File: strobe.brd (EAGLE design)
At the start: 160 x 100 mm, 67 parts, among them IC1 AT90USB162A, Q1 IRF3704S, Q2 IRF3704S, Q4 IRF3704S, Q5 IRF3704S, T1 BC849, T2 BC849, T3 BC849, T4 BC849, T5 BC849, T6 BC849, T7 BC849, T8 BC849, X6 RJ45-6LC21-B

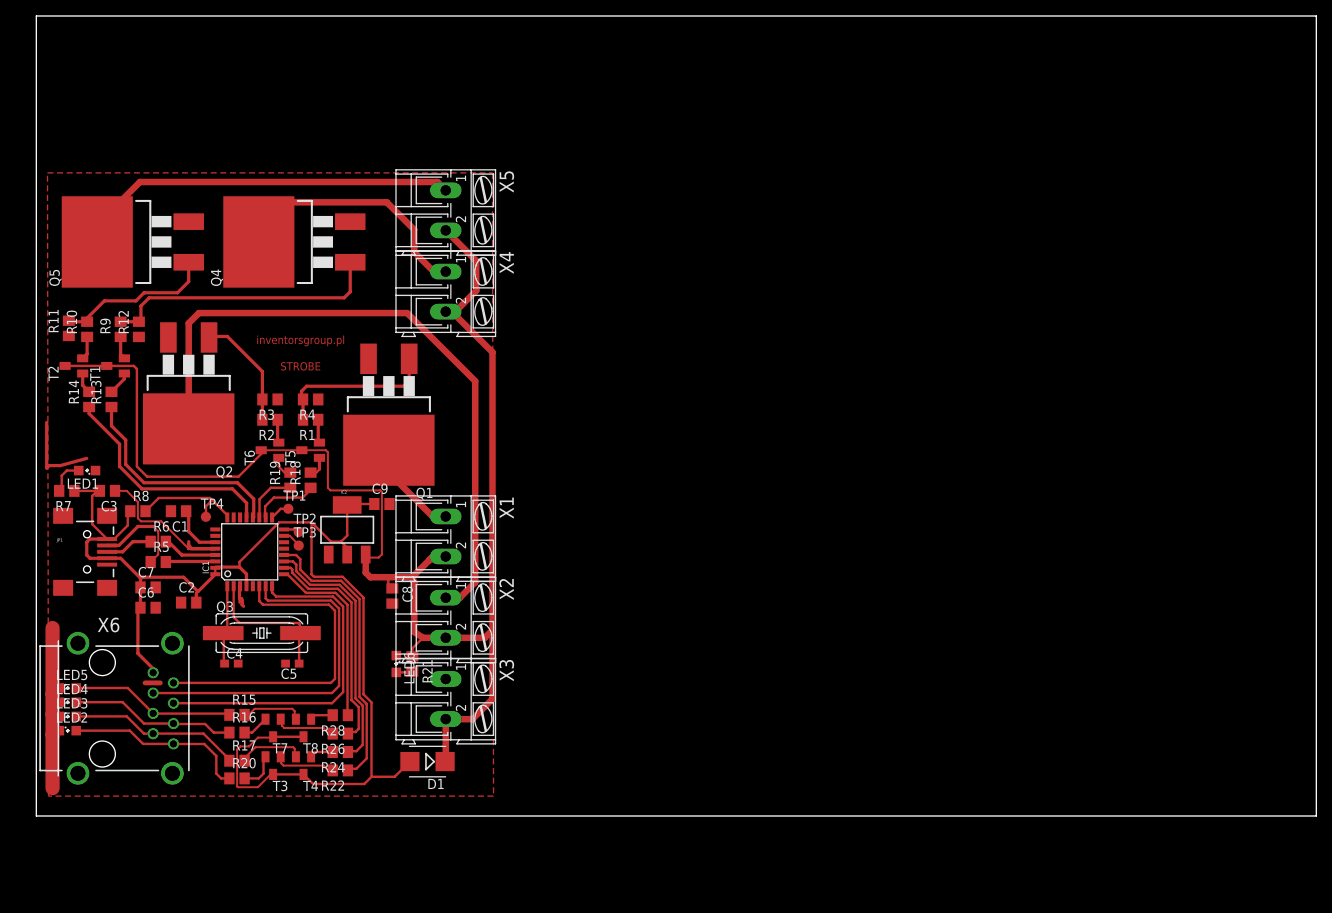
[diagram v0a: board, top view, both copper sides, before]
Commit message: PCB extreme makeover
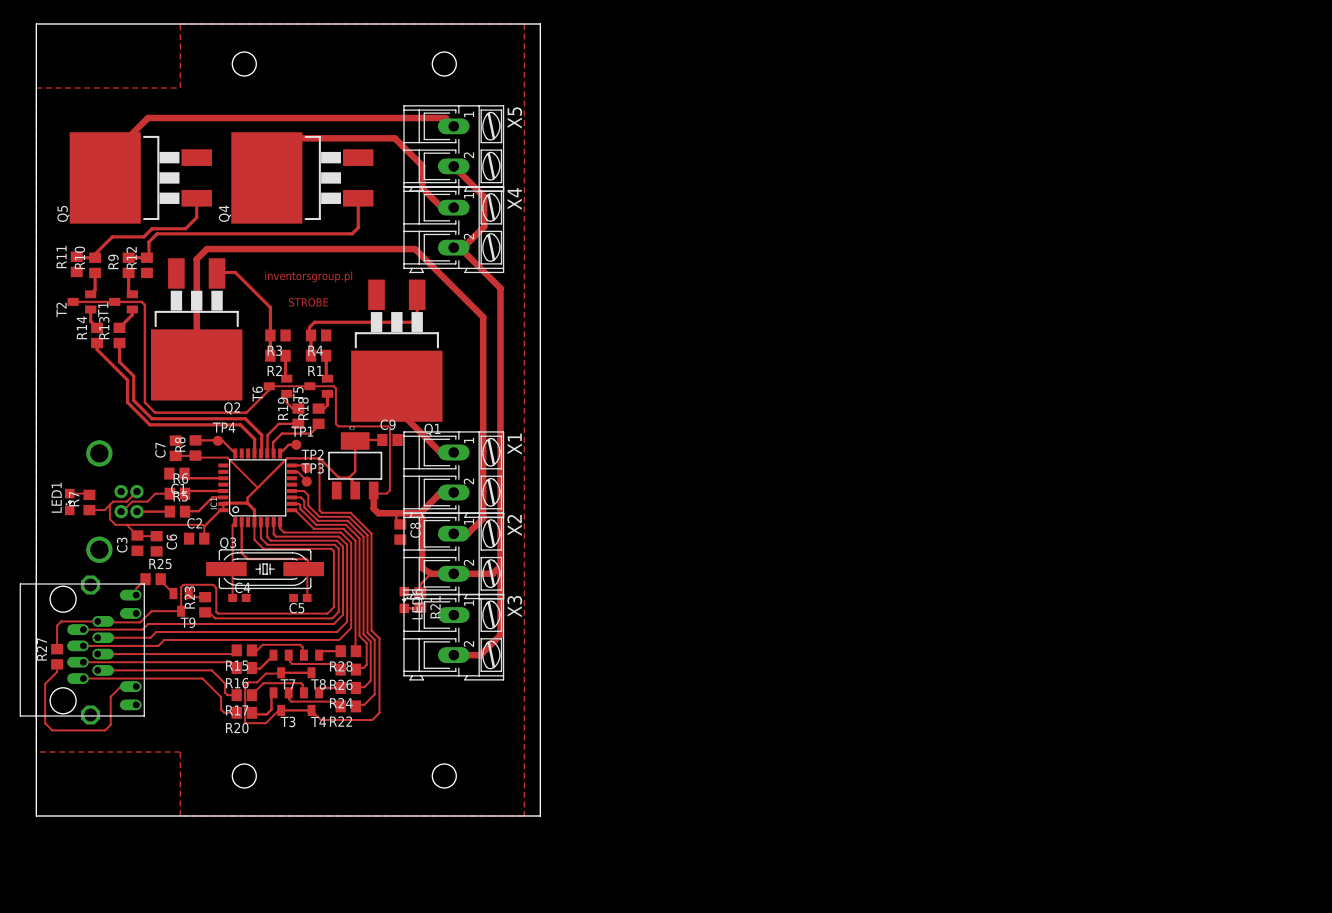
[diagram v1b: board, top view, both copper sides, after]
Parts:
- removed D1: (no value), diode:SMB
- removed LED2, LED3, LED4, LED5: (no value), led:SML0805
- removed X6: RJ45-6LC21-B, con-tycoelectronics:RJ45-SHIELD1
- added R23, R25, R27: (no value), rcl:R0805
- added T9: BC849, transistor:SOT23
- added U$1: RJ45, RJ45:RJ45
- JP1: value USBSMD -> USB-B; device SparkFun-Connectors:USB-MINIB -> SparkFun-Connectors:USB-B-PTH
- moved C7 17.7 mm to (17.4, 46.0), turned to 90 degrees
- moved R8 10.7 mm to (19.9, 46.0), turned to 90 degrees
- moved TP4 9.62 mm to (22.7, 46.9)
- moved C4 8.26 mm to (25.4, 27.2)
- moved C5 8.26 mm to (33.0, 27.2)
- moved R20 8.25 mm to (26.0, 12.9), turned to 180 degrees
- moved R17 8.24 mm to (26.0, 15.1), turned to 180 degrees
- moved R16 8.13 mm to (26.0, 18.5), turned to 180 degrees
- moved R15 8.11 mm to (26.0, 20.7), turned to 180 degrees
- moved C6 8.07 mm to (15.0, 34.0), turned to 270 degrees
- moved Q4 8.06 mm to (31.4, 79.8)
- moved Q5 8.06 mm to (11.2, 79.8)
- moved X5 8.06 mm to (52.2, 83.7)
- moved C9 8.06 mm to (44.2, 47.0)
- moved Q1 8.06 mm to (45.1, 56.3)
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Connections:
- removed net L1: LED2.A, R20.1, X6.8
- removed net L2: LED3.A, R17.1, X6.7
- removed net L3: LED4.A, R16.1, X6.6
- removed net L4: LED5.A, R15.1, X6.5
- new net N$26: R25.1, U$1.L1+
- new net N$33: R15.2, U$1.5
- new net N$35: R16.2, U$1.6
- new net N$36: R17.2, U$1.7
- new net N$38: R20.2, U$1.8
- new net N$39: R23.2, T9.1
- new net N$40: R27.1, U$1.L2+
- new net O5: R25.2, T9.2
- new net T5: IC1.5, R23.1
- net 12V: no longer D1.C
- net 5V: now also R27.2, T9.3, U$1.1; no longer D1.A, X6.1
- net B1: now also U$1.2; no longer X6.2
- net B2: now also U$1.3; no longer X6.3
- net B3: now also U$1.4; no longer X6.4
- net GND: now also U$1.L1-, U$1.L2-; no longer LED2.C, LED3.C, LED4.C, LED5.C, X6.S1, X6.S2, X6.S3, X6.S4
- net O1: now also R20.1; no longer R20.2
- net O2: now also R17.1; no longer R17.2
- net O3: now also R16.1; no longer R16.2
- net O4: now also R15.1; no longer R15.2
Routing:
- net GND: track 67.3 -> 0.03 mm
- net 5V: track 161.2 -> 209.6 mm
- net T5: track 0.00 -> 37.5 mm
- net N$40: track 0.00 -> 24.1 mm
- net L1: track 22.9 -> 0.00 mm
- net N$38: track 0.00 -> 21.8 mm
- net L2: track 21.5 -> 0.00 mm
- net L3: track 20.7 -> 0.00 mm
- net L4: track 20.6 -> 0.00 mm
- net N$35: track 0.00 -> 19.5 mm
- net N$36: track 0.00 -> 19.3 mm
- net N$33: track 0.00 -> 17.6 mm
- net B1: track 40.8 -> 53.6 mm
- net B3: track 42.9 -> 55.5 mm
- net N$14: track 14.5 -> 5.93 mm
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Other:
- board size 160 x 100 mm -> 63 x 99 mm

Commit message: Close-to-final version of board
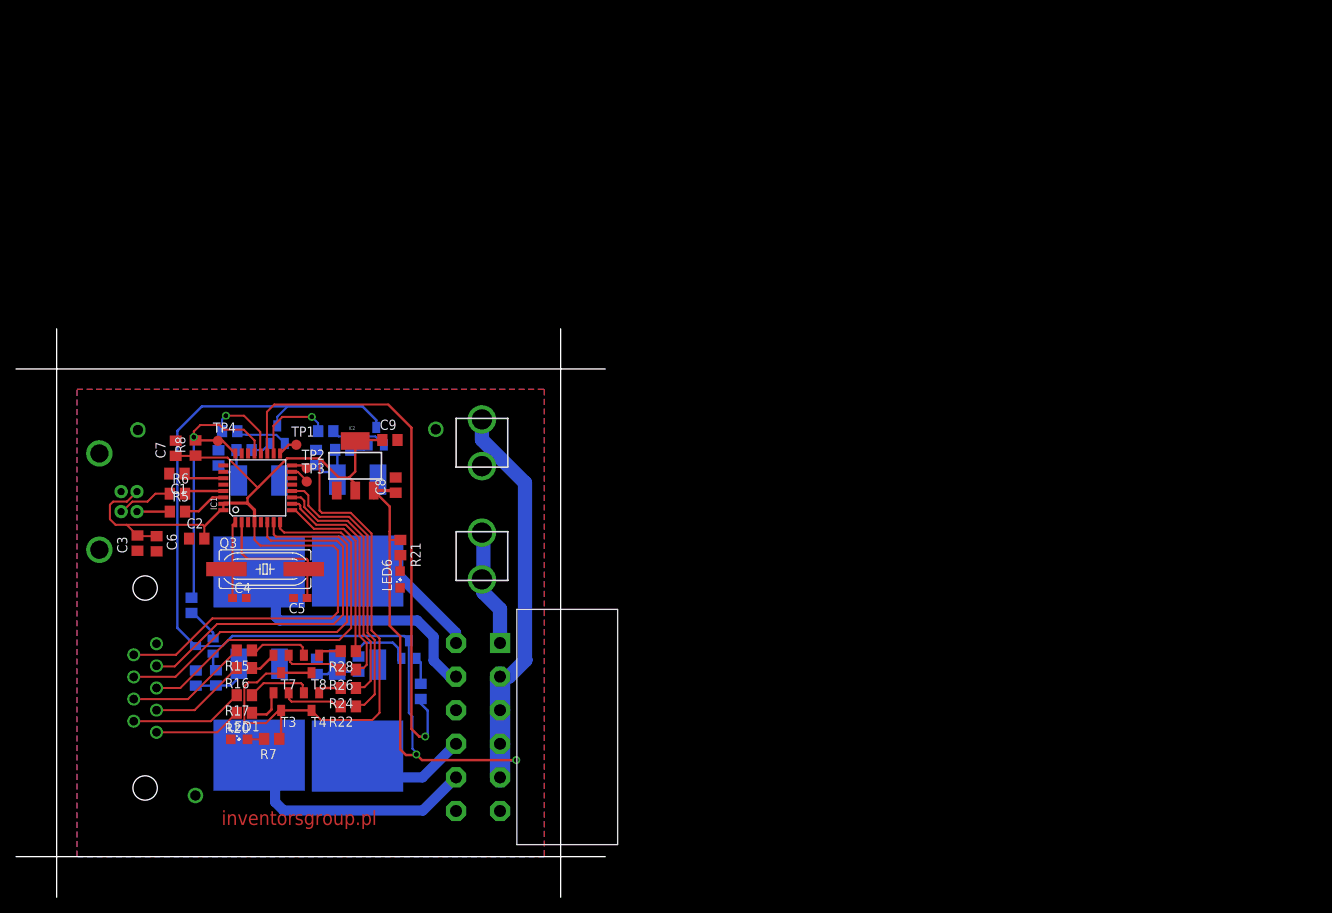
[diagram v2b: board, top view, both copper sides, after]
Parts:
- removed R23, R25, R27: (no value), rcl:R0805
- removed T9: BC849, transistor:SOT23
- removed X1, X2, X3, X4, X5: (no value), con-ptr500:AK300/2
- added F1: FUSEX20MM, SparkFun-Passives:FUSE_5MM
- added X6: D-SUB9-H3M09RA, con-thomas-betts:H3M09RA
- U$1: value RJ45 -> MF42-10; device RJ45:RJ45 -> con-amphenol:MF42-10
- moved Q5 71.6 mm to (27.9, 10.1), flipped to the bottom, turned to 180 degrees
- moved U$1 64.7 mm to (58.0, 4.83), turned to 90 degrees
- moved R11 53.8 mm to (19.9, 17.2), flipped to the bottom, turned to 270 degrees
- moved R10 53.7 mm to (22.4, 17.3), flipped to the bottom, turned to 270 degrees
- moved Q2 52.9 mm to (40.1, 10.0), flipped to the bottom
- moved Q4 46.8 mm to (27.9, 33.0), flipped to the bottom, turned to 180 degrees
- moved T2 45.7 mm to (21.0, 21.2), flipped to the bottom, turned to 270 degrees
- moved R3 41.7 mm to (35.1, 18.7), flipped to the bottom, turned to 270 degrees
- moved R2 39.8 mm to (40.3, 19.0), flipped to the bottom, turned to 270 degrees
- moved R19 37.6 mm to (48.0, 15.6), flipped to the bottom
- moved R7 37.3 mm to (29.4, 9.64), turned to 180 degrees
- moved T6 36.8 mm to (46.6, 20.8), flipped to the bottom, turned to 0 degrees
- moved LED1 36.4 mm to (25.4, 9.59), turned to 0 degrees
- moved R14 35.7 mm to (19.4, 26.3), flipped to the bottom, turned to 270 degrees
- moved R9 27.2 mm to (26.0, 45.7), flipped to the bottom, turned to 0 degrees
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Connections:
- removed net N$16: Q4.2, X4.1
- removed net N$17: Q5.2, X5.1
- removed net N$38: R20.2, U$1.8
- removed net N$39: R23.2, T9.1
- removed net N$4: Q2.2, X2.1
- removed net N$40: R27.1, U$1.L2+
- removed net O5: R25.2, T9.2
- new net L1: Q1.2, U$1.6
- new net L2: Q2.2, U$1.9
- new net L3: Q4.2, U$1.7
- new net L4: Q5.2, U$1.10
- net 12V: now also F1.1, U$1.2, U$1.3, U$1.4, U$1.5; no longer X1.2, X2.2, X3.2, X4.2, X5.2
- net 5V: now also X6.9; no longer R27.2, T9.3, U$1.1
- net B1: now also X6.4; no longer U$1.2
- net B2: now also X6.8; no longer U$1.3
- net B3: now also X6.3; no longer U$1.4
- net GND: now also U$1.11, U$1.12, U$1.8, X6.5; no longer U$1.L1-, U$1.L2-, X3.1
- net N$26: now also R20.2, X6.1; no longer R25.1, U$1.L1+
- net N$3: now also F1.3, U$1.1; no longer Q1.2, X1.1
- net N$33: now also R17.2, X6.6; no longer R15.2, U$1.5
- net N$35: now also X6.2; no longer U$1.6
- net N$36: now also R15.2, X6.7; no longer R17.2, U$1.7
- net T5: no longer R23.1
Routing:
- net N$4: track 89.2 -> 0.00 mm
- net CH2: track 6.77 -> 69.8 mm, vias 0 -> 1
- net N$17: track 48.4 -> 0.00 mm
- net T5: track 37.5 -> 0.00 mm
- net 12V: track 180.5 -> 216.7 mm, vias 0 -> 2
- net L3: track 0.00 -> 33.8 mm
- net L4: track 0.00 -> 31.4 mm
- net N$16: track 31.4 -> 0.00 mm
- net N$11: track 35.3 -> 6.51 mm
- net N$40: track 24.1 -> 0.00 mm
- net N$38: track 21.8 -> 0.00 mm
- net CH3: track 28.1 -> 9.99 mm, vias 0 -> 1
- net L1: track 0.00 -> 16.8 mm
- net 5V: track 209.6 -> 193.9 mm
- net L2: track 0.00 -> 15.2 mm
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- added copper zone on layer 16, net GND
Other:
- board size 63 x 99 mm -> 73.7 x 71.1 mm
- board text removed: "STROBE"
